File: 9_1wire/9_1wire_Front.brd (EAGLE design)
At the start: 71.5 x 24 mm, 2 parts

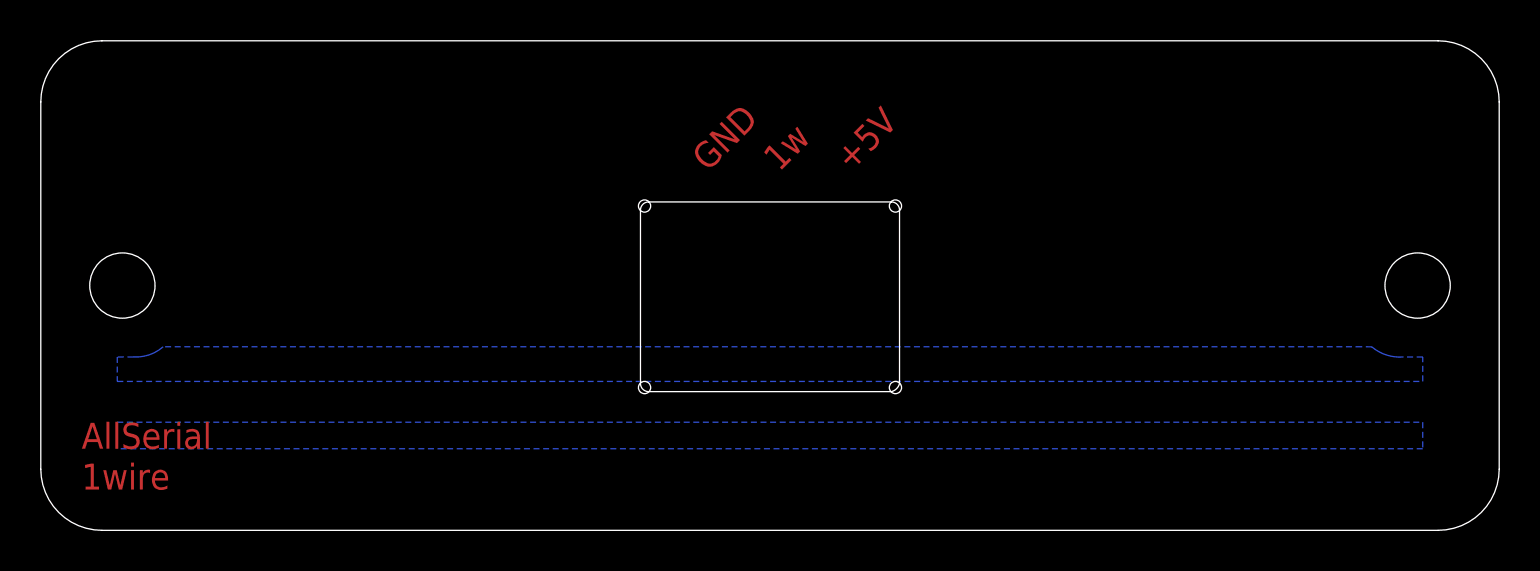
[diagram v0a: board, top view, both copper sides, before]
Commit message: Cleanup, front with lib elements
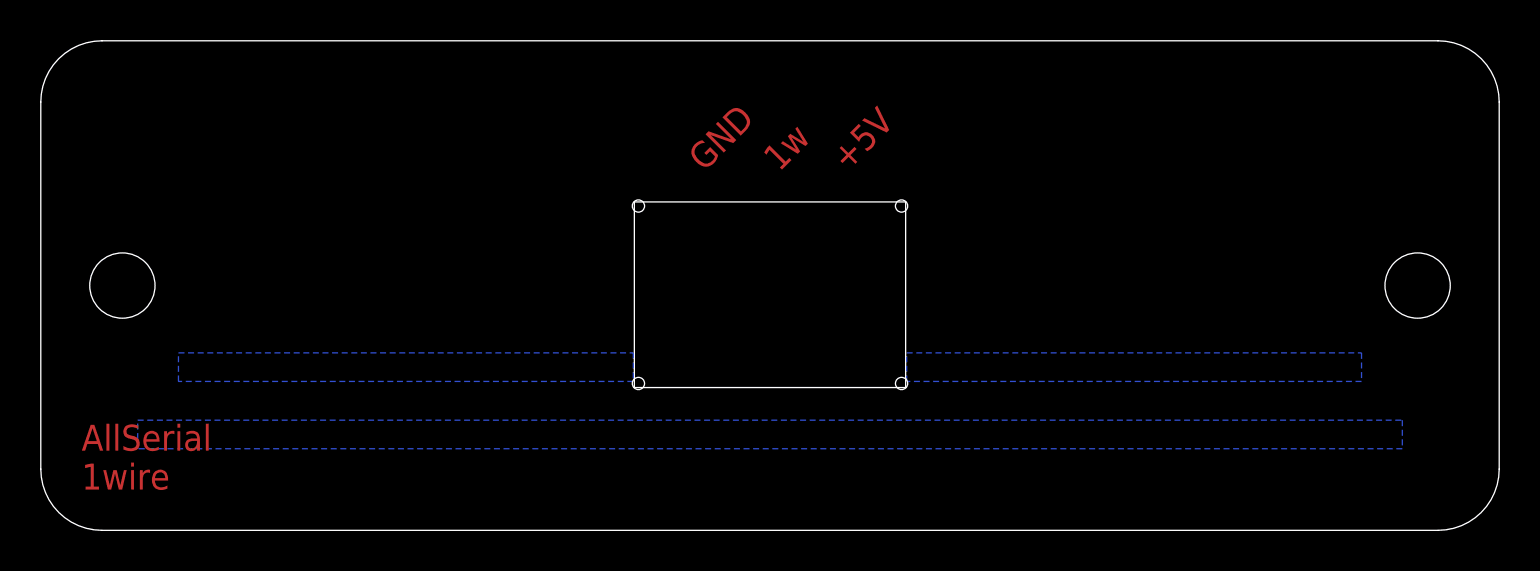
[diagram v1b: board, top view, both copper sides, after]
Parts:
- removed E$1: (no value), AllSerialv2:RIA_AKL182-03
- removed E$2: (no value), AllSerialv2:PANEL
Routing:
- removed copper zone on layer 16, net S$2
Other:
- outline, holes or cut-outs redrawn
- board text added: "AllSerial 1wire"
- board text removed: "1wire"
